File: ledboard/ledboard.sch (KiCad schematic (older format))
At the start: 51 parts, among them J1 LEFT, J2 PWR_L, J3 RIGHT, J4 PWR_R, J5 Conn_01x03_Male, J6 Conn_01x03_Male, J7 Conn_01x02_Male, K1 FINDER-40.31, Q1 BC547, U1 AL8860, U2 AL8860, U3 LM22676MR-5, U4 RASPBERRYPI4_4GB

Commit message: last
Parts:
- removed D10: D, Diode_THT:D_5KP_P10.16mm_Horizontal, symbol Device:D
- removed J6: Conn_01x03_Male, Connector_PinHeader_1.00mm:PinHeader_1x03_P1.00mm_Vertical, symbol Connector:Conn_01x03_Male
- removed J7: Conn_01x02_Male, Connector_PinHeader_1.00mm:PinHeader_1x02_P1.00mm_Vertical, symbol Connector:Conn_01x02_Male
- removed K1: FINDER-40.31, Relay_THT:Relay_SPDT_Finder_40.31, symbol Relay:FINDER-40.31
- removed Q1: BC547, Package_TO_SOT_THT:TO-92_Inline, symbol Transistor_BJT:BC547
- added J6: Conn_01x02_Male, Connector_PinHeader_1.00mm:PinHeader_1x02_P1.00mm_Vertical, symbol Connector:Conn_01x02_Male
- added J8: Conn_01x02_Shielded, Connector:TE_282837-2, symbol Connector_Generic_Shielded:Conn_01x02_Shielded
- added M1: MPMOS, Package_TO_SOT_THT:TO-220-3_Vertical, symbol pspice:MPMOS
- C10: P/N (none) -> VJ0805Y105KXQTW1BC
- C11: P/N (none) -> GRM2195C1H113JA01D
- C12: P/N (none) -> UPJ1A181MED1TD
- C7: P/N (none) -> JMK212ABJ226MG-T
- C8, C9: P/N (none) -> CGA4J3X7S1A685K125AB
- D9: P/N (none) -> CCS15S30,L3QUF
- L3: P/N (none) -> MLZ1608M4R7WT000
- R10: P/N (none) -> Y16291K00000B9R
- R12: value 1k -> 10k; footprint Resistor_SMD:R_0603_1608Metric_Pad1.05x0.95mm_HandSolder -> Resistor_SMD:R_0805_2012Metric_Pad1.15x1.40mm_HandSolder; P/N (none) -> RK73H2ATTE1002F
- R13: value 1k -> 150; footprint Resistor_SMD:R_0603_1608Metric_Pad1.05x0.95mm_HandSolder -> Resistor_SMD:R_0805_2012Metric_Pad1.15x1.40mm_HandSolder; P/N (none) -> CPF0805B150RE1
- R9: P/N (none) -> Y16297K00000B9W
- U4: footprint MODULE_RASPBERRYPI4_4GB -> KiCad raspberry pi:MODULE_RASPBERRYPI4_4GB; symbol RASPBERRYPI4_4GB:RASPBERRYPI4_4GB -> ledboard-rescue:RASPBERRYPI4_4GB-RASPBERRYPI4_4GB
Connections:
- net labels removed: 5V
- wire segments 195 -> 172
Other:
- moved on the sheet: C10, C11, C12, C7, C8, C9, D9, L3, R10, R11, R9, U3

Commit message: hole
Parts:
- R10: P/N Y16291K00000B9R -> RNCP0805FTD1K00
- R11: P/N (none) -> ERA-3AEB1541V
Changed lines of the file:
@@
 F 2 "Resistor_SMD:R_0603_1608Metric_Pad1.05x0.95mm_HandSolder" V 10280 1400 50  0001 C CNN
 F 3 "~" H 10350 1400 50  0001 C CNN
-F 4 "Y16291K00000B9R" V 10350 1400 50  0001 C CNN "P/N"
+F 4 "RNCP0805FTD1K00" V 10350 1400 50  0001 C CNN "P/N"
 	1    10350 1400
 	0    1    1    0
@@
 F 2 "Resistor_SMD:R_0603_1608Metric_Pad1.05x0.95mm_HandSolder" V 10280 1650 50  0001 C CNN
 F 3 "~" H 10350 1650 50  0001 C CNN
+F 4 "ERA-3AEB1541V" H 10350 1650 50  0001 C CNN "P/N"
 	1    10350 1650
 	1    0    0    -1

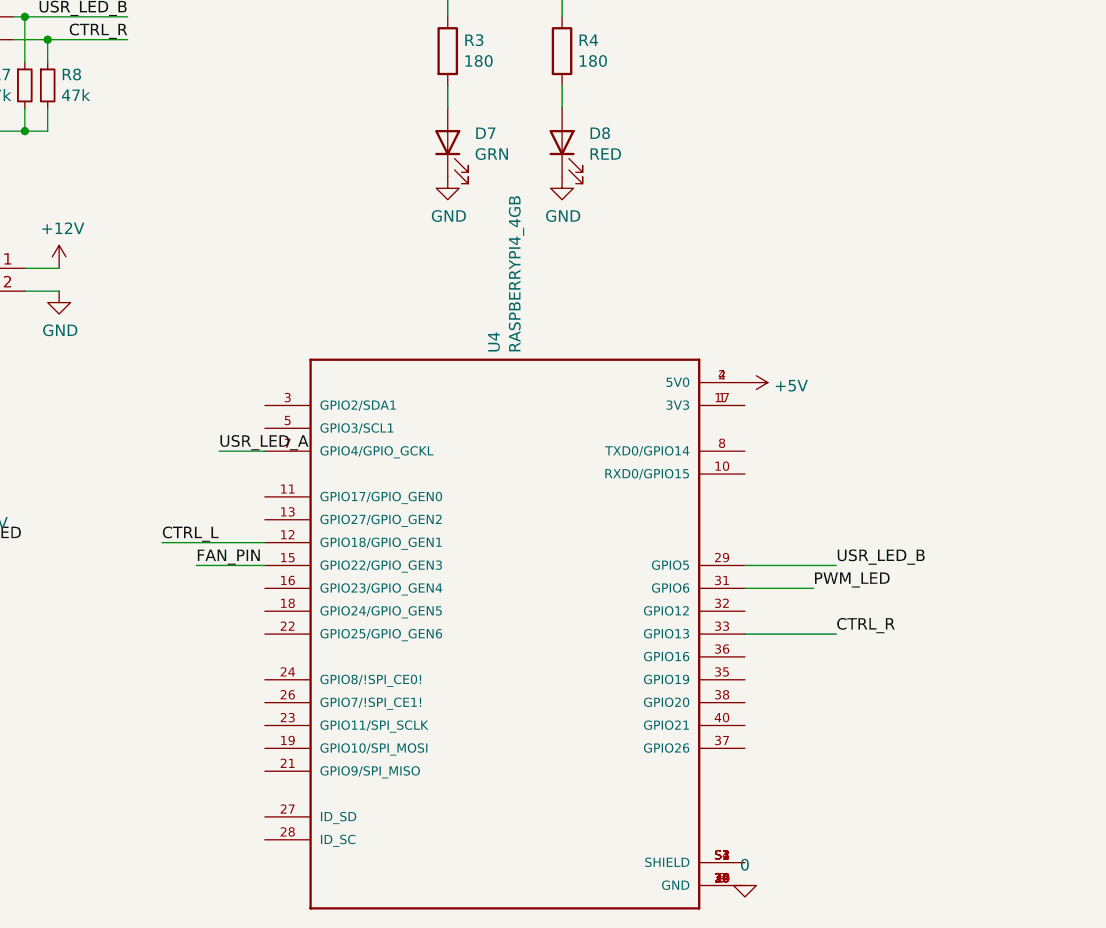
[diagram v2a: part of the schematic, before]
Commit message: wire
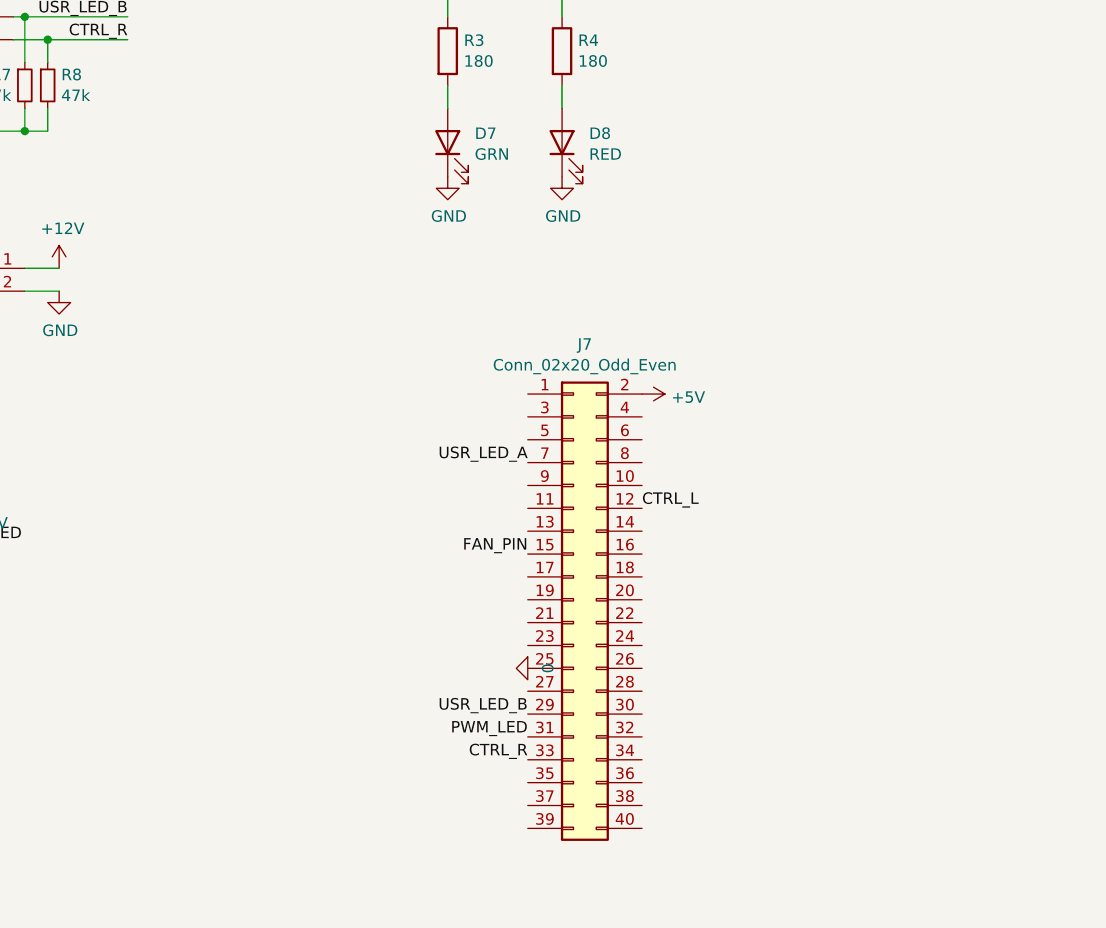
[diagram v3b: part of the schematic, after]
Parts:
- removed U4: RASPBERRYPI4_4GB, KiCad raspberry pi:MODULE_RASPBERRYPI4_4GB, symbol ledboard-rescue:RASPBERRYPI4_4GB-RASPBERRYPI4_4GB
- added J7: Conn_02x20_Odd_Even, Connector_PinHeader_2.54mm:PinHeader_2x20_P2.54mm_Vertical, symbol Connector_Generic:Conn_02x20_Odd_Even
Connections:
- net +5V: now also J7.2 (Pin_2)
- net 0: now also J7.25 (Pin_25)
- net CTRL_L: now also J7.12 (Pin_12)
- net CTRL_R: now also J7.33 (Pin_33)
- net FAN_PIN: now also J7.15 (Pin_15)
- net PWM_LED: now also J7.31 (Pin_31)
- net USR_LED_A: now also J7.7 (Pin_7)
- net USR_LED_B: now also J7.29 (Pin_29)
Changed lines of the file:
@@
 	1    0    0    -1
 $EndComp
-$Comp
-L ledboard-rescue:RASPBERRYPI4_4GB-RASPBERRYPI4_4GB U4
-U 1 1 5F62C8C9
-P 5150 6200
-F 0 "U4" V 5054 7230 50  0000 L CNN
-F 1 "RASPBERRYPI4_4GB" V 5145 7230 50  0000 L CNN
-F 2 "KiCad raspberry pi:MODULE_RASPBERRYPI4_4GB" H 5150 6200 50  0001 L BNN
-F 3 "Manufacturer Recommendations" H 5150 6200 50  0001 L BNN
-F 4 "18mm" H 5150 6200 50  0001 L BNN "Field4"
-F 5 "Raspberry Pi" H 5150 6200 50  0001 L BNN "Field5"
-F 6 "1.0" H 5150 6200 50  0001 L BNN "Field6"
-	1    5150 6200
-	1    0    0    -1
-$EndComp
-Wire Wire Line
-	3850 5600 4050 5600
-Text Label 3850 5600 0    50   ~ 0
+Text Label 5200 5650 2    50   ~ 0
 USR_LED_A
-Wire Wire Line
-	6150 6100 6550 6100
-Text Label 6550 6100 0    50   ~ 0
-USR_LED_B
-Wire Wire Line
-	6150 6400 6550 6400
-Text Label 6550 6400 0    50   ~ 0
+Text Label 5200 6950 2    50   ~ 0
 CTRL_R
-Wire Wire Line
-	4050 6000 3600 6000
-Text Label 3600 6000 0    50   ~ 0
+Text Label 5700 5850 0    50   ~ 0
 CTRL_L
 $Comp
@@
 PWM_LED
 Wire Wire Line
-	6150 6200 6450 6200
-Text Label 6450 6200 0    50   ~ 0
-PWM_LED
-Wire Wire Line
 	2300 5800 2350 5800
 Wire Wire Line
@@
 	1    0    0    -1
 $EndComp
-Wire Wire Line
-	3750 6100 4050 6100
-Text Label 3750 6100 0    50   ~ 0
+Text Label 5200 6050 2    50   ~ 0
 FAN_PIN
 Wire Wire Line
@@
 	7550 1650 7550 1700
 $Comp
-L power:+5V #PWR0101
-U 1 1 5F9E449F
-P 6150 5300
-F 0 "#PWR0101" H 6150 5150 50  0001 C CNN
-F 1 "+5V" V 6165 5428 50  0000 L CNN
-F 2 "" H 6150 5300 50  0001 C CNN
-F 3 "" H 6150 5300 50  0001 C CNN
-	1    6150 5300
-	0    1    1    0
-$EndComp
-$Comp
 L power:+12V #PWR0102
 U 1 1 5F9E5194
@@
 L pspice:0 #GND0108
 U 1 1 5FA2B309
-P 6150 7500
-F 0 "#GND0108" H 6150 7400 50  0001 C CNN
-F 1 "0" H 6150 7589 50  0000 C CNN
-F 2 "" H 6150 7500 50  0001 C CNN
-F 3 "~" H 6150 7500 50  0001 C CNN
-	1    6150 7500
-	1    0    0    -1
+P 5200 6550
+F 0 "#GND0108" H 5200 6450 50  0001 C CNN
+F 1 "0" H 5200 6639 50  0000 C CNN
+F 2 "" H 5200 6550 50  0001 C CNN
+F 3 "~" H 5200 6550 50  0001 C CNN
+	1    5200 6550
+	0    1    1    0
 $EndComp
 $Comp
@@
 	-1   0    0    1
 $EndComp
+Text Label 5200 6850 2    50   ~ 0
+PWM_LED
+Text Label 5200 6750 2    50   ~ 0
+USR_LED_B
+$Comp
+L power:+5V #PWR0101
+U 1 1 5F9E449F
+P 5700 5350
+F 0 "#PWR0101" H 5700 5200 50  0001 C CNN
+F 1 "+5V" V 5715 5478 50  0000 L CNN
+F 2 "" H 5700 5350 50  0001 C CNN
+F 3 "" H 5700 5350 50  0001 C CNN
+	1    5700 5350
+	0    1    1    0
+$EndComp
+$Comp
+L Connector_Generic:Conn_02x20_Odd_Even J7
+U 1 1 5FD76DDB
+P 5400 6250
+F 0 "J7" H 5450 7367 50  0000 C CNN
+F 1 "Conn_02x20_Odd_Even" H 5450 7276 50  0000 C CNN
+F 2 "Connector_PinHeader_2.54mm:PinHeader_2x20_P2.54mm_Vertical" H 5400 6250 50  0001 C CNN
+F 3 "~" H 5400 6250 50  0001 C CNN
+	1    5400 6250
+	1    0    0    -1
+$EndComp
 $EndSCHEMATC

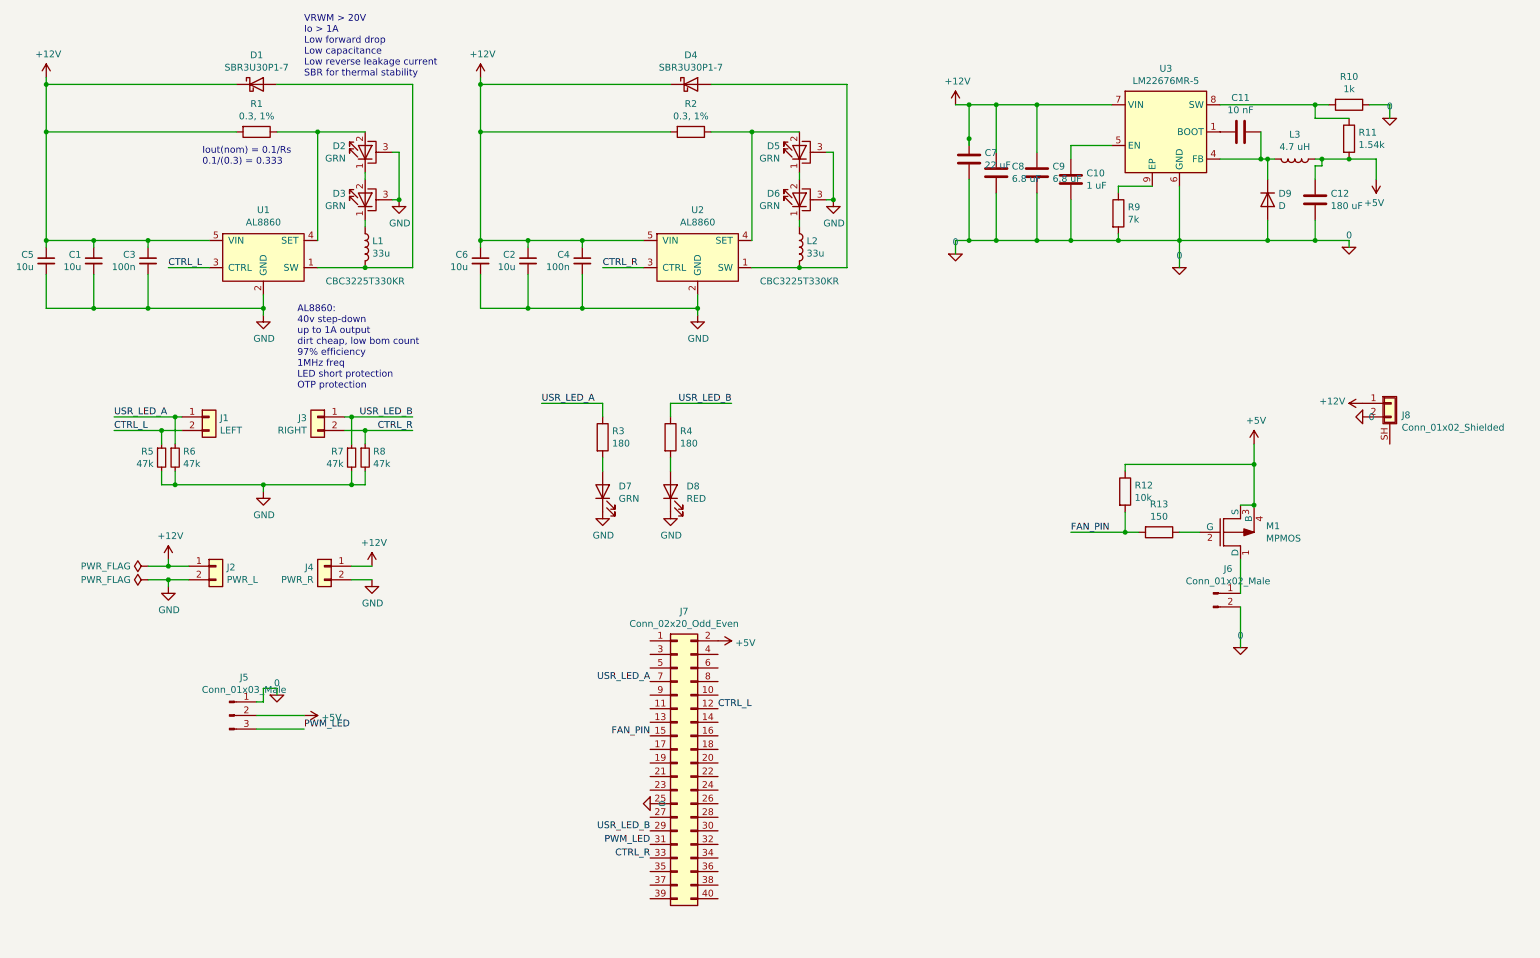
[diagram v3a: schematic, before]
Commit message: Umarım son olur
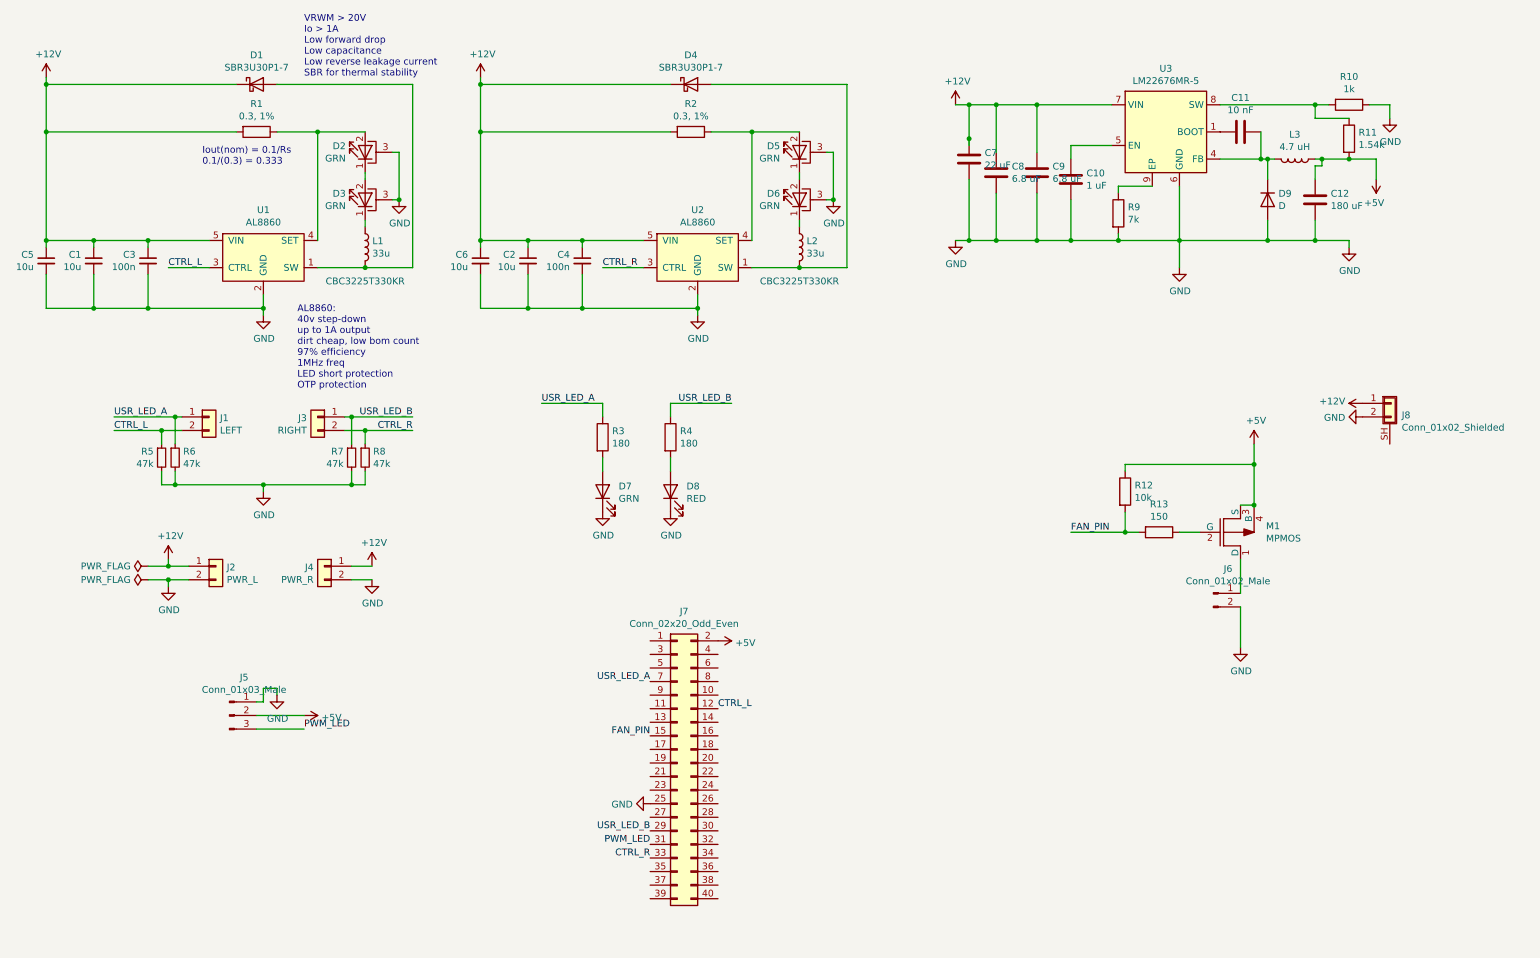
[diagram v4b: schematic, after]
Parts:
- J5: footprint Connector_PinHeader_1.00mm:PinHeader_1x03_P1.00mm_Vertical -> Connector_PinHeader_1.00mm:PinHeader_1x03_P1.00mm_Horizontal
- J6: footprint Connector_PinHeader_1.00mm:PinHeader_1x02_P1.00mm_Vertical -> Connector_PinHeader_1.00mm:PinHeader_1x02_P1.00mm_Horizontal
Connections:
- net 0 is gone; now on net GND: C10.2, C12.2, C7.2, C8.2, C9.2, D9.2 (A), J5.1 (Pin_1), J6.2 (Pin_2), J7.25 (Pin_25), J8.2 (Pin_2), R10.1, R9.2, U3.6 (GND)
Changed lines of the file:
@@
 Wire Wire Line
 	10350 1800 10550 1800
-$Comp
-L pspice:0 #GND0101
-U 1 1 5F7D466C
-P 9100 2600
-F 0 "#GND0101" H 9100 2500 50  0001 C CNN
-F 1 "0" H 9100 2689 50  0000 C CNN
-F 2 "" H 9100 2600 50  0001 C CNN
-F 3 "~" H 9100 2600 50  0001 C CNN
-	1    9100 2600
-	1    0    0    -1
-$EndComp
 Wire Wire Line
 	10650 1400 10650 1500
-$Comp
-L pspice:0 #GND0102
-U 1 1 5F7DB7DF
-P 10650 1500
-F 0 "#GND0102" H 10650 1400 50  0001 C CNN
-F 1 "0" H 10650 1589 50  0000 C CNN
-F 2 "" H 10650 1500 50  0001 C CNN
-F 3 "~" H 10650 1500 50  0001 C CNN
-	1    10650 1500
-	1    0    0    -1
-$EndComp
 Wire Wire Line
 	10350 2400 10350 2450
-$Comp
-L pspice:0 #GND0103
-U 1 1 5F7E15A3
-P 10350 2450
-F 0 "#GND0103" H 10350 2350 50  0001 C CNN
-F 1 "0" H 10350 2539 50  0000 C CNN
-F 2 "" H 10350 2450 50  0001 C CNN
-F 3 "~" H 10350 2450 50  0001 C CNN
-	1    10350 2450
-	1    0    0    -1
-$EndComp
-$Comp
-L pspice:0 #GND0104
-U 1 1 5F7E204A
-P 7450 2500
-F 0 "#GND0104" H 7450 2400 50  0001 C CNN
-F 1 "0" H 7450 2589 50  0000 C CNN
-F 2 "" H 7450 2500 50  0001 C CNN
-F 3 "~" H 7450 2500 50  0001 C CNN
-	1    7450 2500
-	1    0    0    -1
-$EndComp
-Wire Wire Line
-	7450 2500 7450 2400
 $Comp
 L Device:C C12
@@
 F 0 "J5" H 2208 6181 50  0000 C CNN
 F 1 "Conn_01x03_Male" H 2208 6090 50  0000 C CNN
-F 2 "Connector_PinHeader_1.00mm:PinHeader_1x03_P1.00mm_Vertical" H 2100 5900 50  0001 C CNN
+F 2 "Connector_PinHeader_1.00mm:PinHeader_1x03_P1.00mm_Horizontal" H 2100 5900 50  0001 C CNN
 F 3 "~" H 2100 5900 50  0001 C CNN
 	1    2100 5900
@@
 Wire Wire Line
 	2450 5700 2450 5750
-$Comp
-L pspice:0 #GND0105
-U 1 1 5F6A7CF3
-P 2450 5750
-F 0 "#GND0105" H 2450 5650 50  0001 C CNN
-F 1 "0" H 2450 5839 50  0000 C CNN
-F 2 "" H 2450 5750 50  0001 C CNN
-F 3 "~" H 2450 5750 50  0001 C CNN
-	1    2450 5750
-	1    0    0    -1
-$EndComp
 Text Label 5200 6050 2    50   ~ 0
 FAN_PIN
@@
 FAN_PIN
 $Comp
-L pspice:0 #GND0106
-U 1 1 5F9AAF30
-P 9550 5400
-F 0 "#GND0106" H 9550 5300 50  0001 C CNN
-F 1 "0" H 9550 5489 50  0000 C CNN
-F 2 "" H 9550 5400 50  0001 C CNN
-F 3 "~" H 9550 5400 50  0001 C CNN
-	1    9550 5400
-	1    0    0    -1
-$EndComp
-$Comp
 L Connector:Conn_01x02_Male J6
 U 1 1 5F9BE96D
@@
 F 0 "J6" H 9458 5181 50  0000 C CNN
 F 1 "Conn_01x02_Male" H 9458 5090 50  0000 C CNN
-F 2 "Connector_PinHeader_1.00mm:PinHeader_1x02_P1.00mm_Vertical" H 9350 5000 50  0001 C CNN
+F 2 "Connector_PinHeader_1.00mm:PinHeader_1x02_P1.00mm_Horizontal" H 9350 5000 50  0001 C CNN
 F 3 "~" H 9350 5000 50  0001 C CNN
 	1    9350 5000
@@
 	1    0    0    -1
 $EndComp
-$Comp
-L pspice:0 #GND0107
-U 1 1 5F9DA70B
-P 10450 3700
-F 0 "#GND0107" H 10450 3600 50  0001 C CNN
-F 1 "0" V 10450 3744 50  0000 L CNN
-F 2 "" H 10450 3700 50  0001 C CNN
-F 3 "~" H 10450 3700 50  0001 C CNN
-	1    10450 3700
-	0    1    1    0
-$EndComp
 Wire Wire Line
 	7550 1400 7550 1650
@@
 $EndComp
 $Comp
-L pspice:0 #GND0108
-U 1 1 5FA2B309
-P 5200 6550
-F 0 "#GND0108" H 5200 6450 50  0001 C CNN
-F 1 "0" H 5200 6639 50  0000 C CNN
-F 2 "" H 5200 6550 50  0001 C CNN
-F 3 "~" H 5200 6550 50  0001 C CNN
-	1    5200 6550
-	0    1    1    0
-$EndComp
-$Comp
 L power:+5V #PWR0110
 U 1 1 5FA33C77
@@
 	1    0    0    -1
 $EndComp
+$Comp
+L power:GND #PWR0111
+U 1 1 5FD8A76C
+P 2450 5750
+F 0 "#PWR0111" H 2450 5500 50  0001 C CNN
+F 1 "GND" H 2455 5577 50  0000 C CNN
+F 2 "" H 2450 5750 50  0001 C CNN
+F 3 "" H 2450 5750 50  0001 C CNN
+	1    2450 5750
+	1    0    0    -1
+$EndComp
+$Comp
+L power:GND #PWR0112
+U 1 1 5FD8B108
+P 5200 6550
+F 0 "#PWR0112" H 5200 6300 50  0001 C CNN
+F 1 "GND" V 5205 6422 50  0000 R CNN
+F 2 "" H 5200 6550 50  0001 C CNN
+F 3 "" H 5200 6550 50  0001 C CNN
+	1    5200 6550
+	0    1    1    0
+$EndComp
+$Comp
+L power:GND #PWR0113
+U 1 1 5FD999FC
+P 9550 5400
+F 0 "#PWR0113" H 9550 5150 50  0001 C CNN
+F 1 "GND" H 9555 5227 50  0000 C CNN
+F 2 "" H 9550 5400 50  0001 C CNN
+F 3 "" H 9550 5400 50  0001 C CNN
+	1    9550 5400
+	1    0    0    -1
+$EndComp
+$Comp
+L power:GND #PWR0114
+U 1 1 5FDA13DE
+P 10450 3700
+F 0 "#PWR0114" H 10450 3450 50  0001 C CNN
+F 1 "GND" V 10455 3572 50  0000 R CNN
+F 2 "" H 10450 3700 50  0001 C CNN
+F 3 "" H 10450 3700 50  0001 C CNN
+	1    10450 3700
+	0    1    1    0
+$EndComp
+$Comp
+L power:GND #PWR0115
+U 1 1 5FDAF109
+P 7450 2400
+F 0 "#PWR0115" H 7450 2150 50  0001 C CNN
+F 1 "GND" H 7455 2227 50  0000 C CNN
+F 2 "" H 7450 2400 50  0001 C CNN
+F 3 "" H 7450 2400 50  0001 C CNN
+	1    7450 2400
+	1    0    0    -1
+$EndComp
+$Comp
+L power:GND #PWR0116
+U 1 1 5FDB60C0
+P 9100 2600
+F 0 "#PWR0116" H 9100 2350 50  0001 C CNN
+F 1 "GND" H 9105 2427 50  0000 C CNN
+F 2 "" H 9100 2600 50  0001 C CNN
+F 3 "" H 9100 2600 50  0001 C CNN
+	1    9100 2600
+	1    0    0    -1
+$EndComp
+$Comp
+L power:GND #PWR0117
+U 1 1 5FDBD030
+P 10350 2450
+F 0 "#PWR0117" H 10350 2200 50  0001 C CNN
+F 1 "GND" H 10355 2277 50  0000 C CNN
+F 2 "" H 10350 2450 50  0001 C CNN
+F 3 "" H 10350 2450 50  0001 C CNN
+	1    10350 2450
+	1    0    0    -1
+$EndComp
+$Comp
+L power:GND #PWR0118
+U 1 1 5FDC40F4
+P 10650 1500
+F 0 "#PWR0118" H 10650 1250 50  0001 C CNN
+F 1 "GND" H 10655 1327 50  0000 C CNN
+F 2 "" H 10650 1500 50  0001 C CNN
+F 3 "" H 10650 1500 50  0001 C CNN
+	1    10650 1500
+	1    0    0    -1
+$EndComp
